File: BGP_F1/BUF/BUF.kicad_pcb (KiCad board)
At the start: 2 copper layers, 28 x 24 mm, 21 parts, among them P1 CONN_01X02, P2 CONN_01X05, P3 CONN_01X12, U1 MC33178

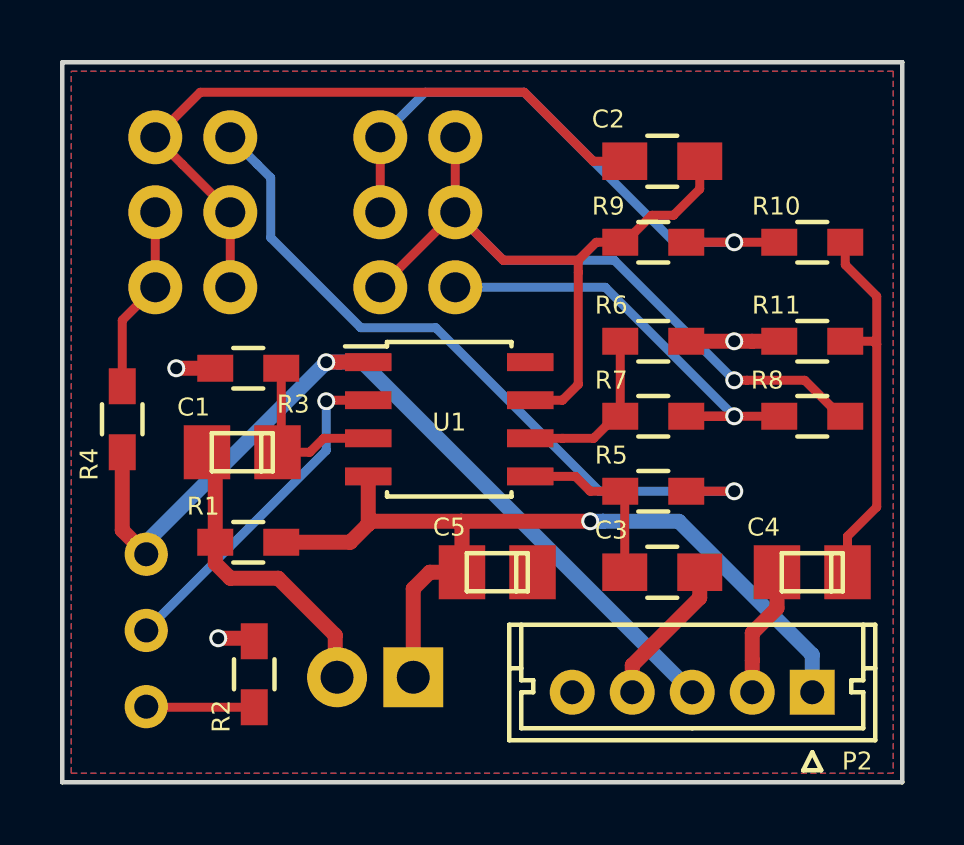
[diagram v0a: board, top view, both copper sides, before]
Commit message: Pot tinkering
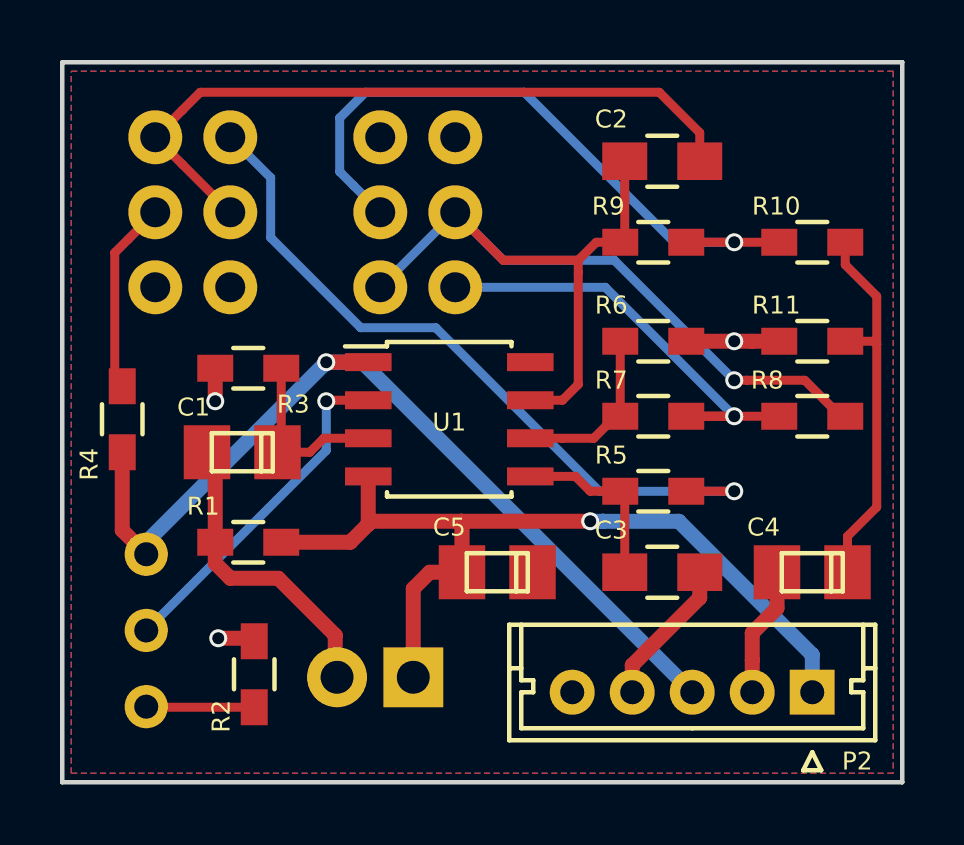
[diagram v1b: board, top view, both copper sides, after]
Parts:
- turned C2 to 180 degrees
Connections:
- P3 pad 12: /PG1_1 -> /PG2_3
- P3 pad 2: /PF1_1 -> /PF1_2
- P3 pad 4: /PF1_3 -> /PF2_1
- P3 pad 9: /PG1_2 -> /PG1_3
- R4 pad 1: /PF1_1 -> /PF1_2
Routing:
- net /PF1_2: track 0.00 -> 6.46 mm
- net /PF1_1: track 6.26 -> 0.00 mm
- net /PG1_1: track 38.5 -> 34.6 mm
- net /PG1_2: track 20.2 -> 22.5 mm
- net /PF1_3: track 23.3 -> 23.8 mm
